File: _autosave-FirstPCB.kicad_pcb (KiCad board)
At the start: 2 copper layers, 77.6 x 38.2 mm, 24 parts, among them SW1 SW_Push, U1 ATmega32U4-AU, Y1 16MHz

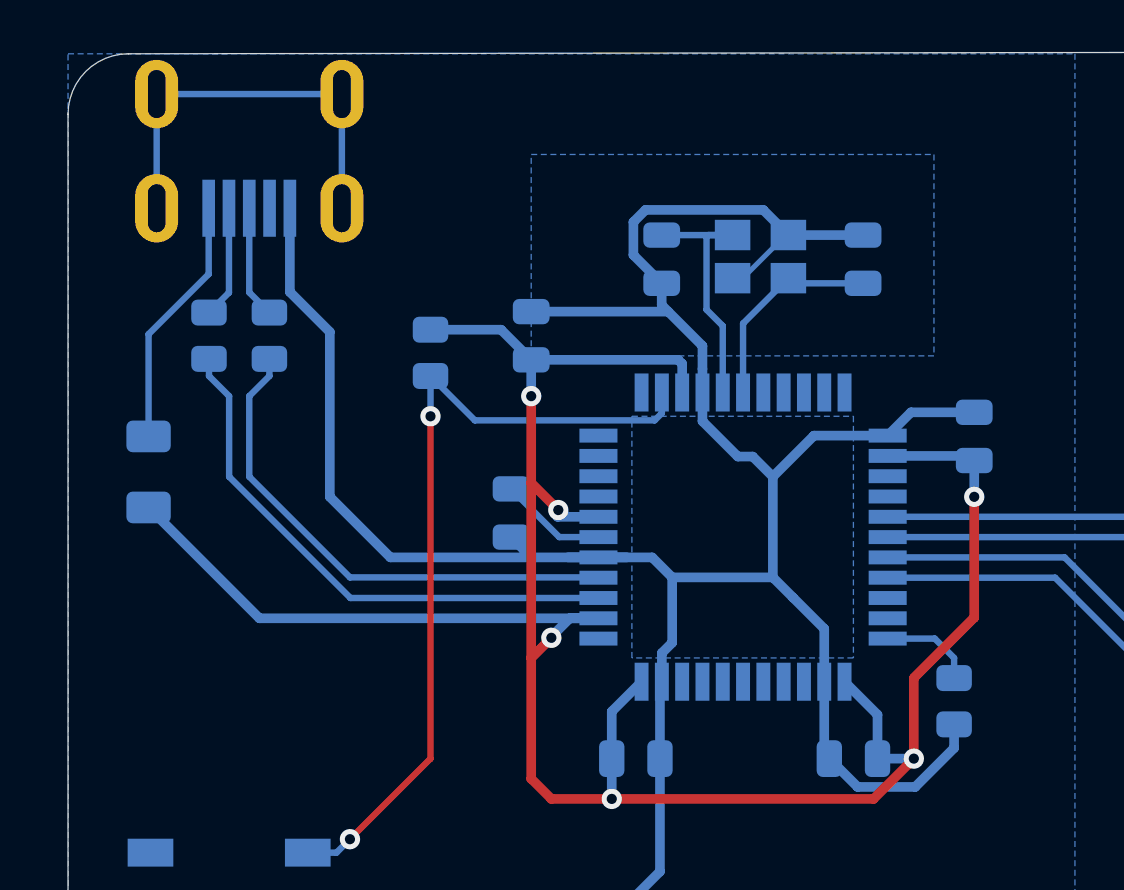
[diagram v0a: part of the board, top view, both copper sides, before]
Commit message: Updates
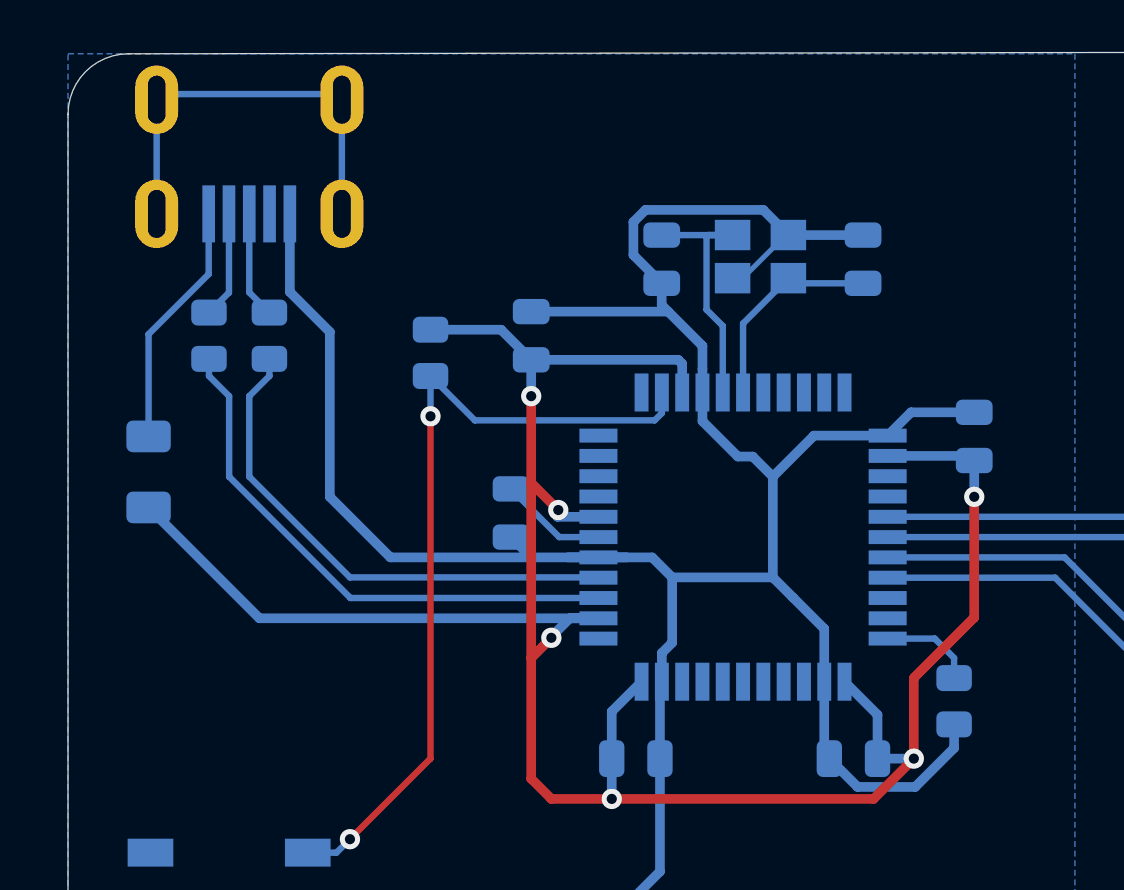
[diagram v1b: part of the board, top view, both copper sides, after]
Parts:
- moved USB1 0.22 mm to (76.2, 109.0)
